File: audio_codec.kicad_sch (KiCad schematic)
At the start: 38 parts, among them J2 AudioOutput, J3 AudioInput, J4 Headphones, U2 WM8731SEDS, U5 TPA6110A2DGN

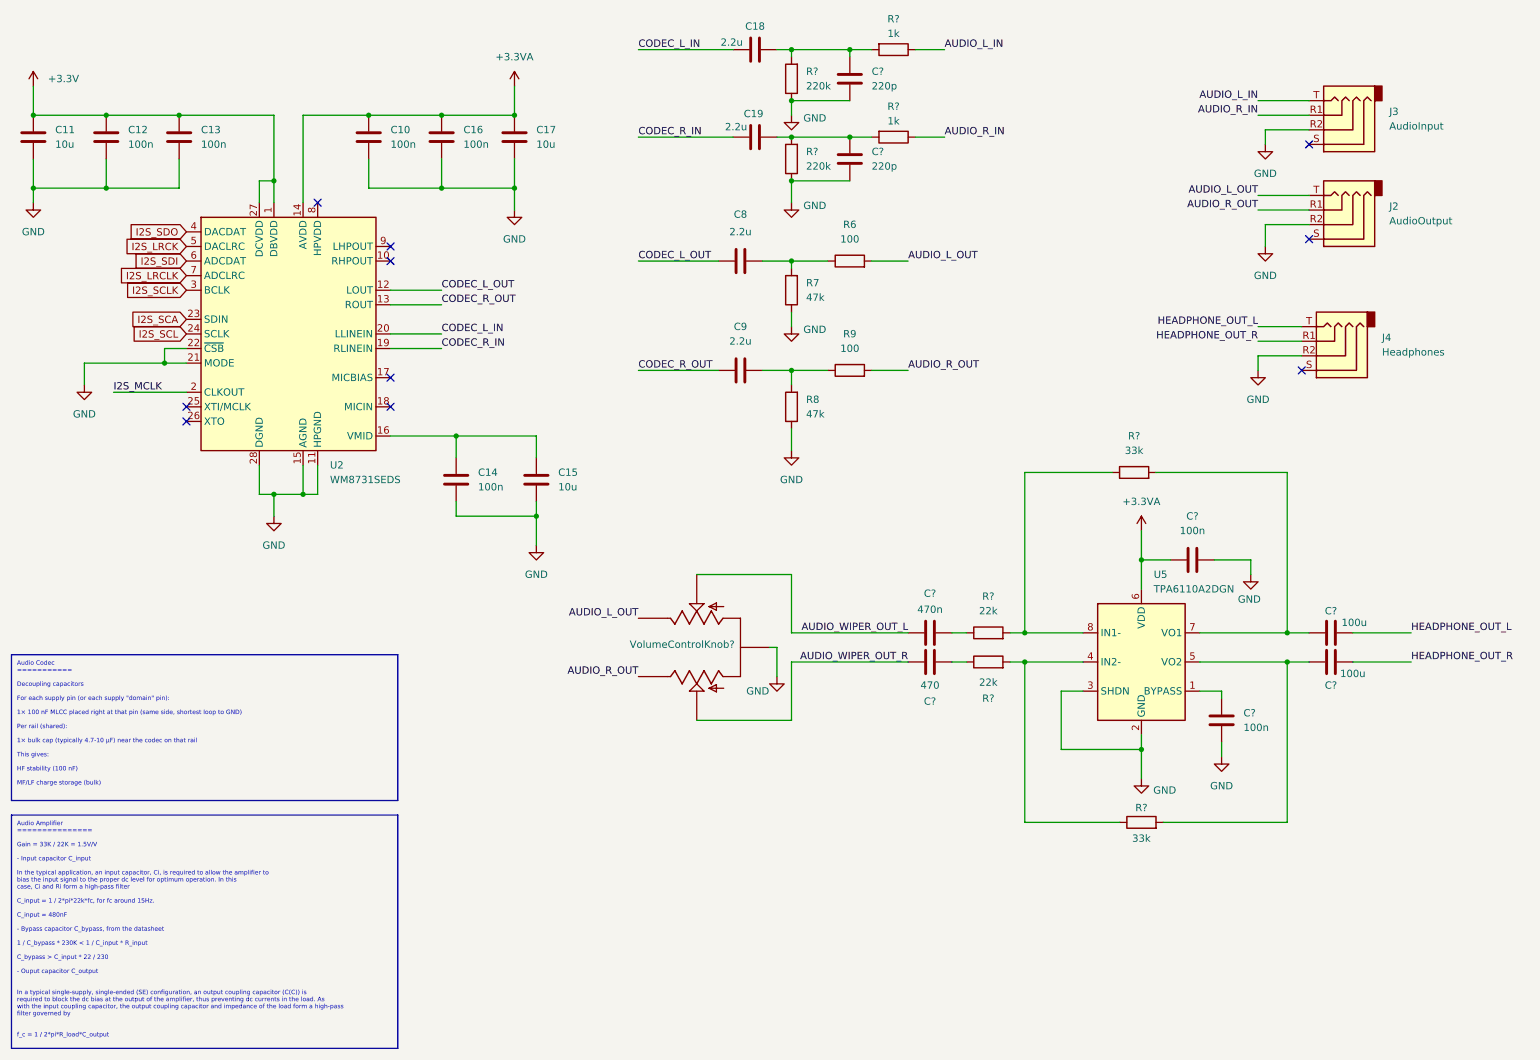
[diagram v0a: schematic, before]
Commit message: First pins assingments
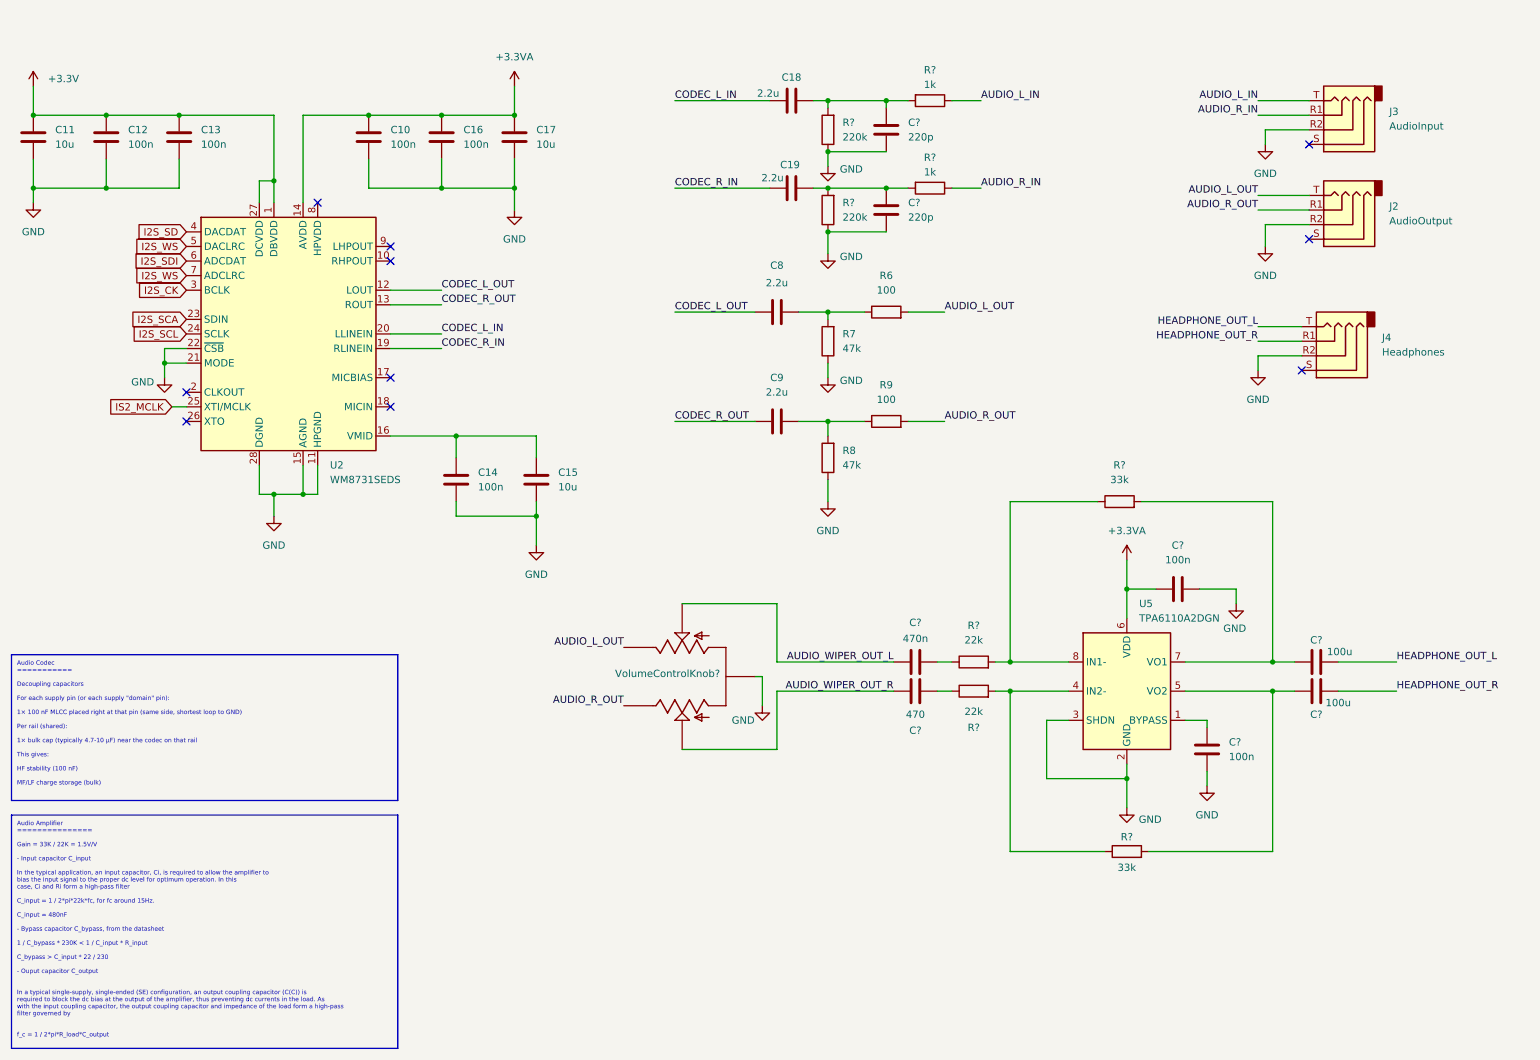
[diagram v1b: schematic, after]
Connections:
- net I2S_LRCLK is gone; now on net I2S_WS: U2.7 (ADCLRC)
- net IS2_MCLK: now reaches U2.25 (XTI/MCLK)
- net I2S_LRCK renamed I2S_WS
- net I2S_MCLK: no longer names the net of U2.2 (CLKOUT)
- net I2S_SCLK renamed I2S_CK
- net I2S_SDO renamed I2S_SD
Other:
- moved on the sheet: C18, C19, C8, C9, C?, R6, R7, R8, R9, R?, U5, VolumeControlKnob?
